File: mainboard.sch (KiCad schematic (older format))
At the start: 77 parts, among them IC1 ATXMEGA128A1U-A, J1 USB, K1 X_MIN, K2 X_MAX, K3 Y_MIN, K4 Y_MAX, K5 Z_MIN, K6 Z_MAX, P1 POWER, P10 USART, P11 TH_HB, P12 TH_EX, P13 TH_HO, P14 LCD, P2 PDI, P3 GPIO_B, P4 BEEPER, P5 OPEN_COLL_D, P6 12V, P7 5V, P8 3.3V, P9 I2C, U1 NE 4558 D SMD, U2 ULN_2003_A

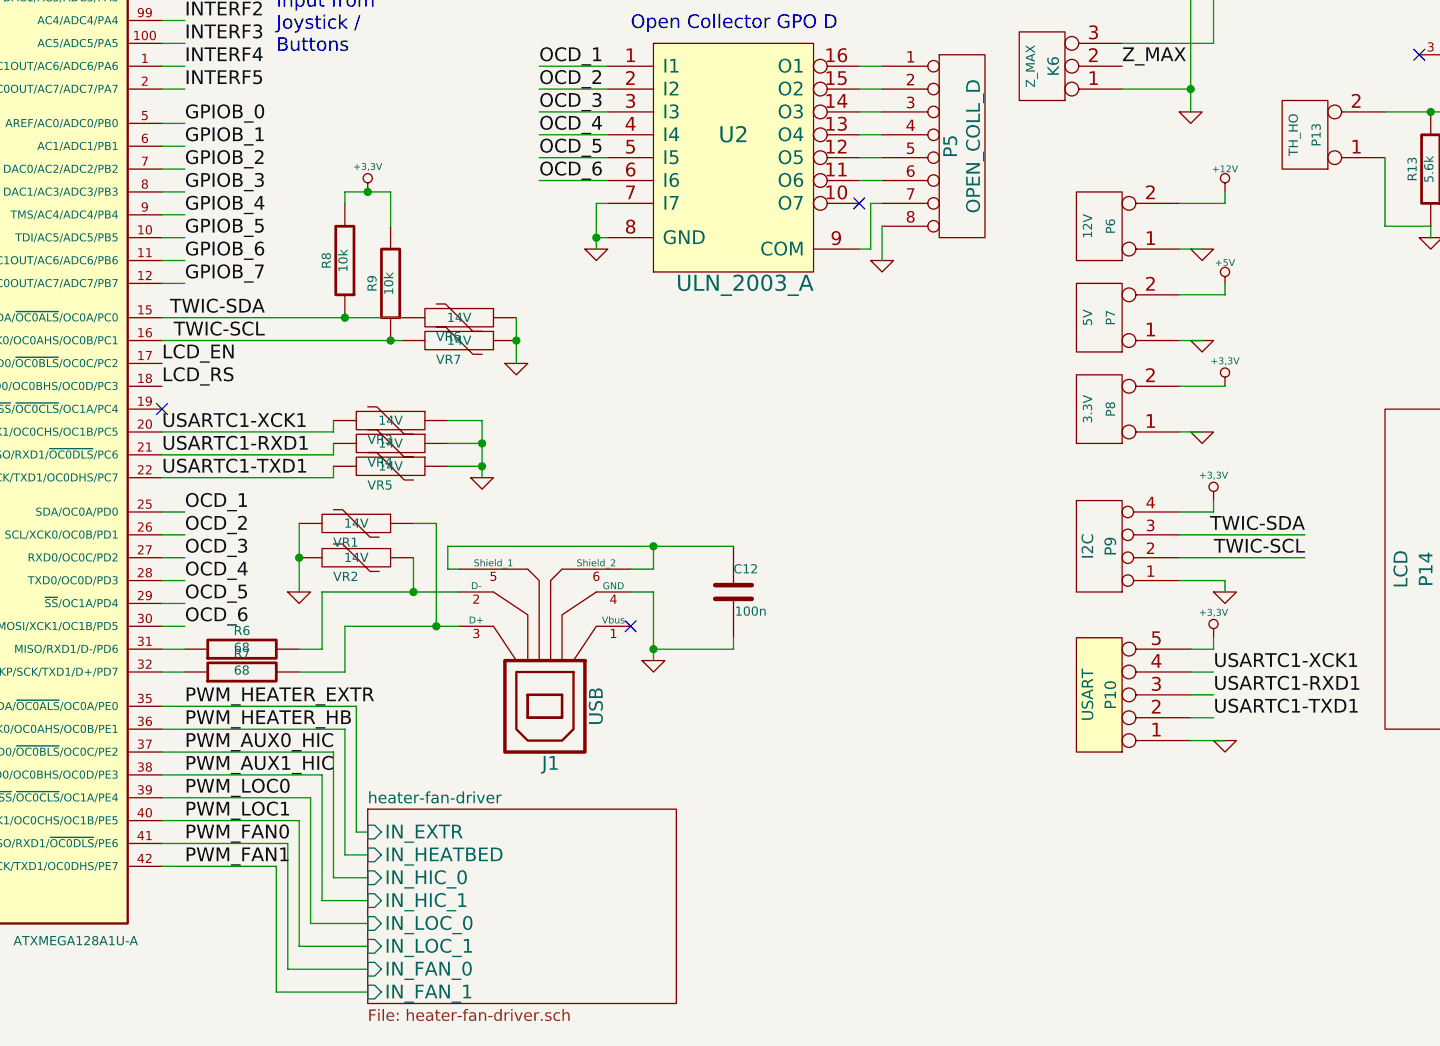
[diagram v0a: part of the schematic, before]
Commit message: Reworked schematic
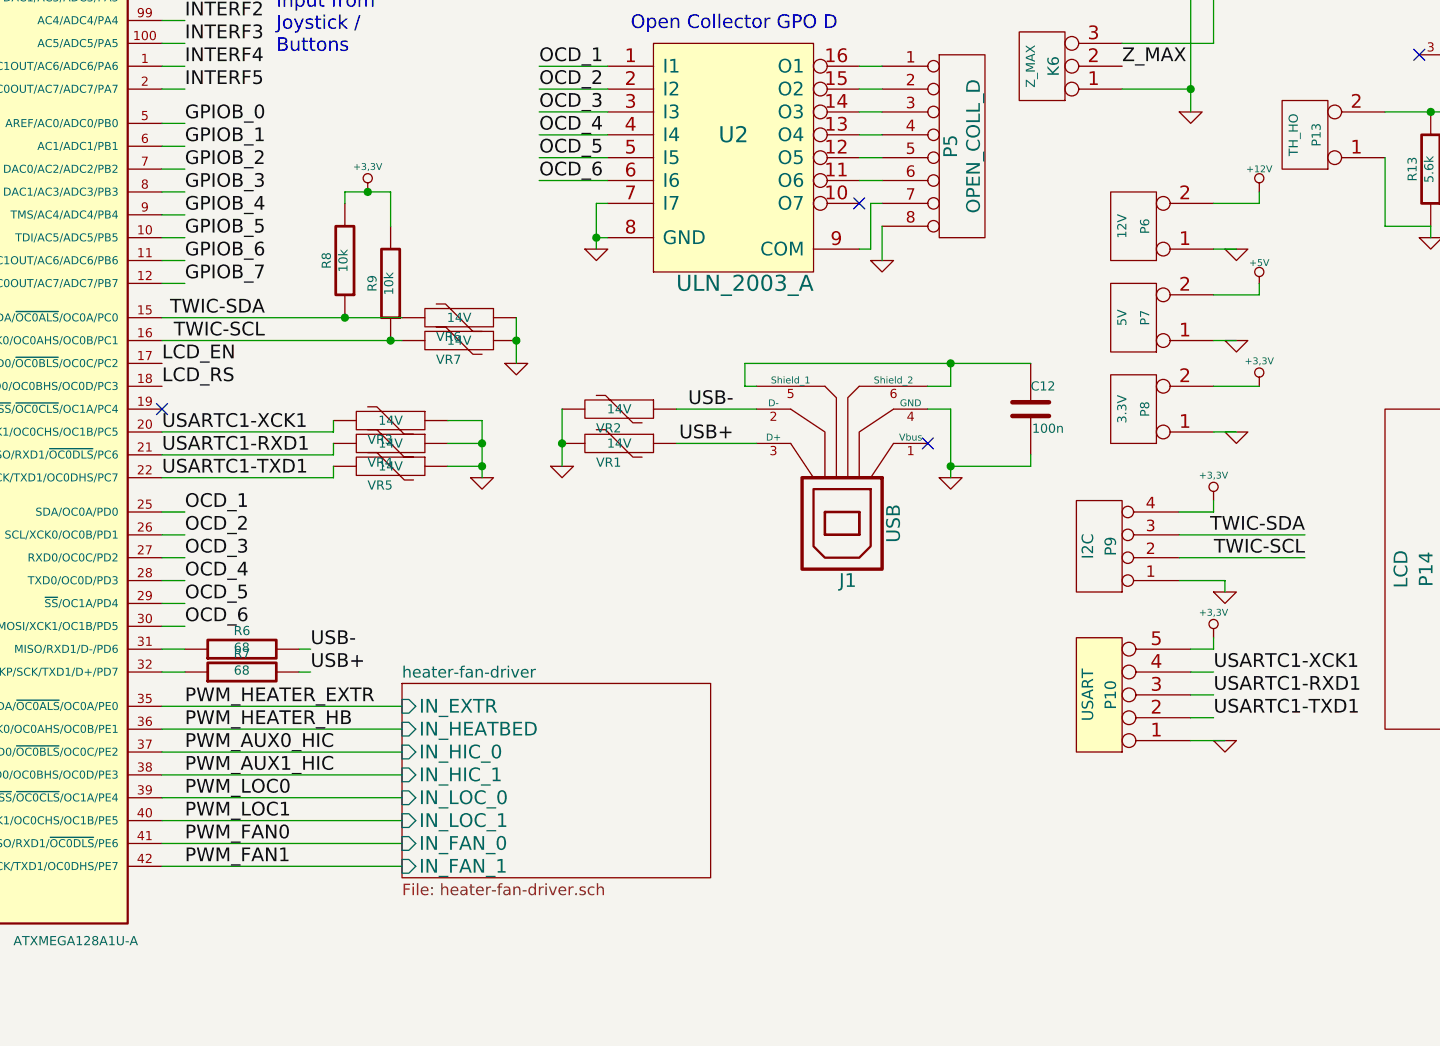
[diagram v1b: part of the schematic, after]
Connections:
- net USB-: now reaches J1.2 (D-), R6.2, VR2.1
- net USB+: now reaches J1.3 (D+), R7.2, VR1.1
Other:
- moved on the sheet: C12, J1, P6, P7, P8, VR1, VR2
